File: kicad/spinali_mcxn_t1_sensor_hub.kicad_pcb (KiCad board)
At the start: 6 copper layers, 45 x 46 mm, 199 parts, among them J1 5055780421, J2 USB4105-GF-A, J3 CAN0A, J4 CAN0B, J5 Debug, J6 CAN1A, J7 CAN1B, J8 DF40TC(3.0)-50DP-0.4V(51), J9 DF40TC(3.0)-50DP-0.4V(51), Q1 BUK6D56-60EX, SW1 SW_SPST, U1 LM74700, U10 BMM350, U11 BMP581, U12 TJA1462ATK, U13 TJA1462ATK, U14 SK9822-EC20, U15 TJA1103AHN, U2 NX5P3363UKZ, U3 LM5160DNTJ, U4 NX5P3363UKZ, U5 MIC5504-1.8YMT, U6 MPM3811GG-Z, U7 MCXN947VDFT, U8 PCMF1USB3SZ, U9 ICM-45686, Y1 24MHz, Y2 32.768kHz, Y3 25MHz

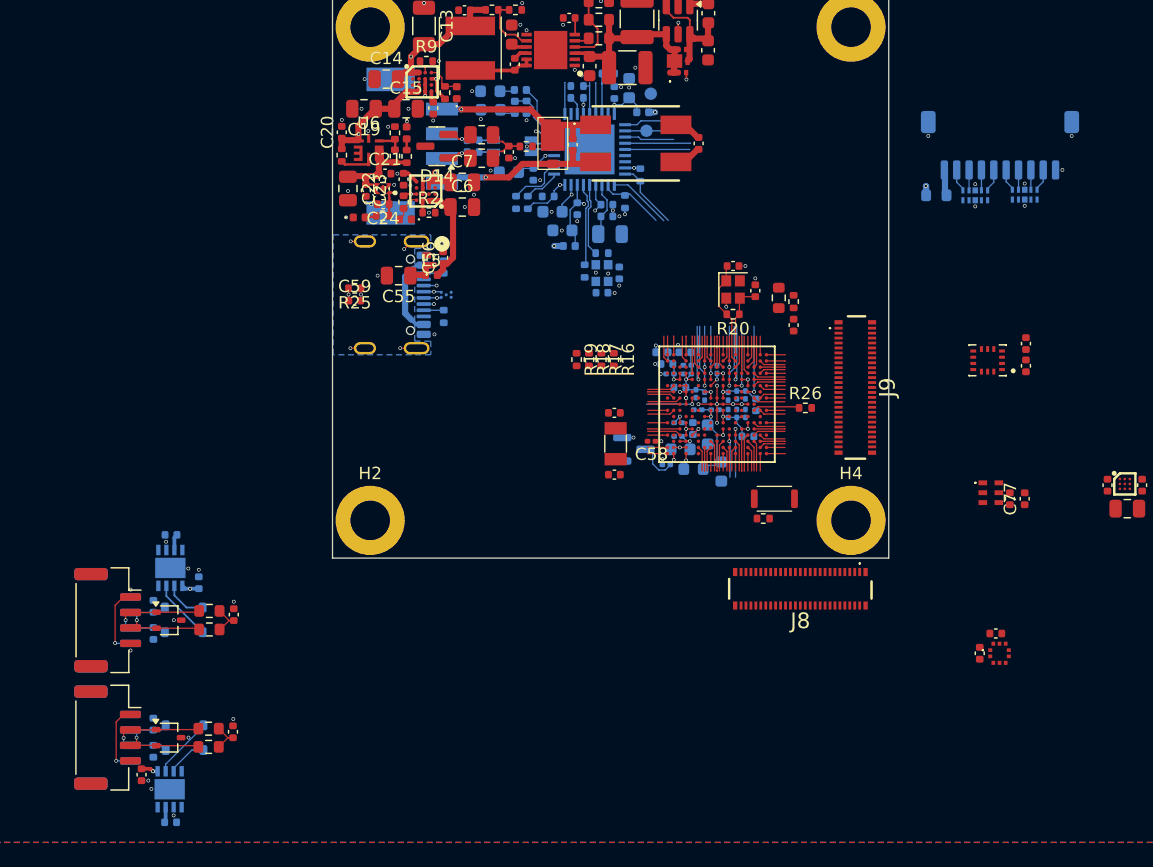
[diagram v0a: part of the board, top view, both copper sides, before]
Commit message: Updated layout
Made layout around CANBUS and USB-C.
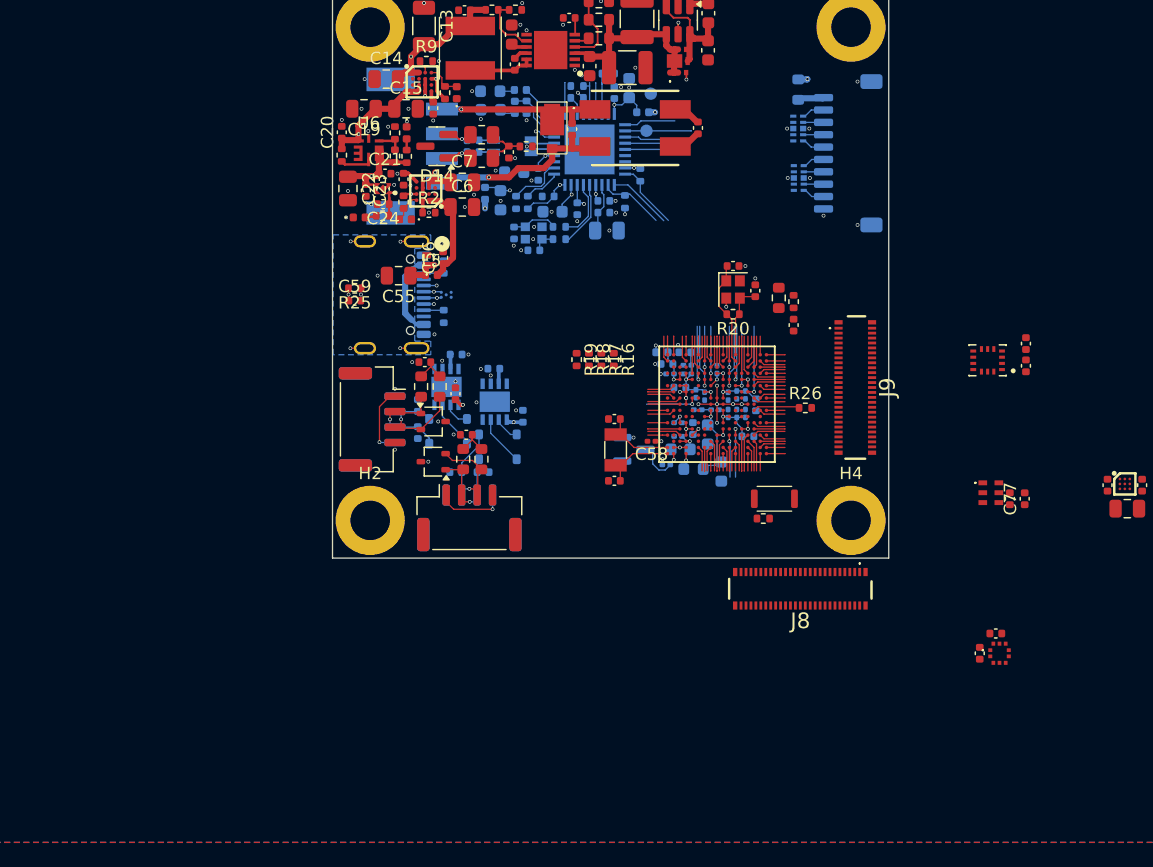
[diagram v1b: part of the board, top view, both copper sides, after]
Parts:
- C67: moved to B.Cu
- C72: moved to F.Cu
- moved C68 45.1 mm to (95.2, 106.7), turned to 180 degrees
- moved C67 42.3 mm to (97.5, 110.5), turned to 90 degrees
- moved U12 40.9 mm to (95.3, 109.3), turned to -90 degrees
- moved C69 35.0 mm to (94.3, 115.0), turned to 0 degrees
- moved L6 34.6 mm to (97.0, 112.0)
- moved J3 34.2 mm to (93.2, 118.8), turned to 180 degrees
- moved J4 34.2 mm to (93.2, 118.8), turned to 0 degrees
- moved R28 32.1 mm to (94.2, 114.0), turned to -90 degrees
- moved C71 31.9 mm to (92.1, 115.0), turned to 0 degrees
- moved D10 30.9 mm to (90.3, 114.2), turned to 180 degrees
- moved C70 30.6 mm to (93.0, 112.0), turned to 0 degrees
- moved R27 30.0 mm to (92.7, 114.0), turned to 90 degrees
- moved C73 27.3 mm to (92.2, 105.5), turned to 0 degrees
- moved R31 27.1 mm to (90.8, 108.1), turned to -90 degrees
- moved C74 26.9 mm to (89.0, 111.8)
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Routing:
- net /Ethernet PHY/VDDA_AO: track 12.8 -> 17.4 mm, vias 2 -> 3
- net /MCU IO Part 2/P5_0/EXTAL32K: track 1.60 -> 6.04 mm
- net /MCU IO Part 2/P5_1/XTAL32K: track 1.60 -> 6.00 mm
- net Net-(C90-Pad1): track 0.00 -> 3.70 mm
- net Net-(U12-CANL): track 4.99 -> 2.09 mm
- net Net-(D10-A2): track 10.8 -> 13.4 mm
- net Net-(D10-A1): track 10.9 -> 8.87 mm, vias 2 -> 1
- net Net-(C91-Pad1): track 0.00 -> 1.87 mm
- net /Ethernet PHY/ENET0_XTAL_IN: track 6.75 -> 4.90 mm
- net Net-(D11-A1): track 10.6 -> 9.19 mm
- net Net-(U13-CANL): track 3.46 -> 2.11 mm
- net Net-(D11-A2): track 10.8 -> 9.75 mm
- net Net-(C1-Pad1): track 14.2 -> 15.2 mm
- net Net-(U13-CANH): track 4.97 -> 3.97 mm
- net Net-(U12-CANH): track 3.26 -> 4.07 mm
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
